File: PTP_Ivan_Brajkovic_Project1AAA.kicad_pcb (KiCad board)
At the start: 2 copper layers, 45 parts, among them J1 Screw_Terminal_01x02, SW1 SW_Push_Dual_x2, SW2 SW2, U1 LM2574N-5, U2 4027, U3 4027, U4 74LS47, U5 FYS-3911BUHR-21, U6 74LVC1G11, U7 NE555P

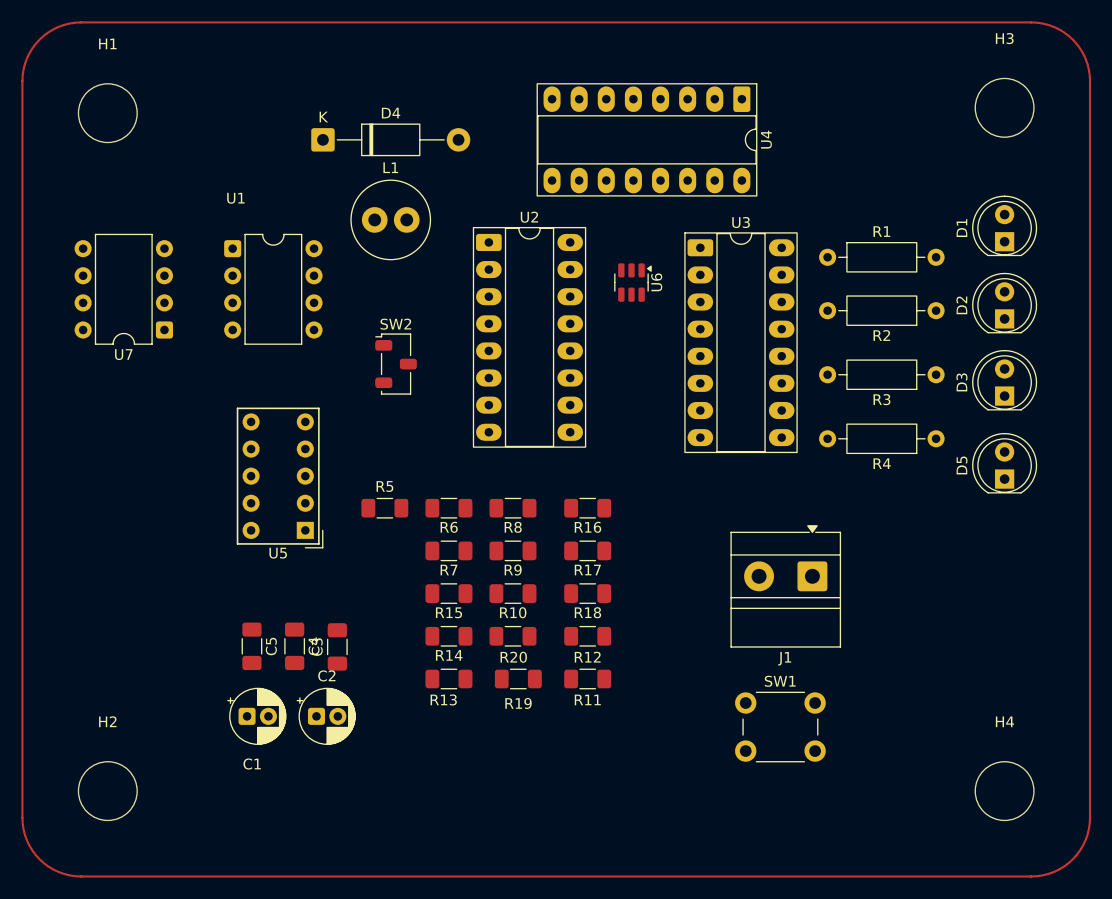
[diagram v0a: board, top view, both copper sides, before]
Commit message: lv7
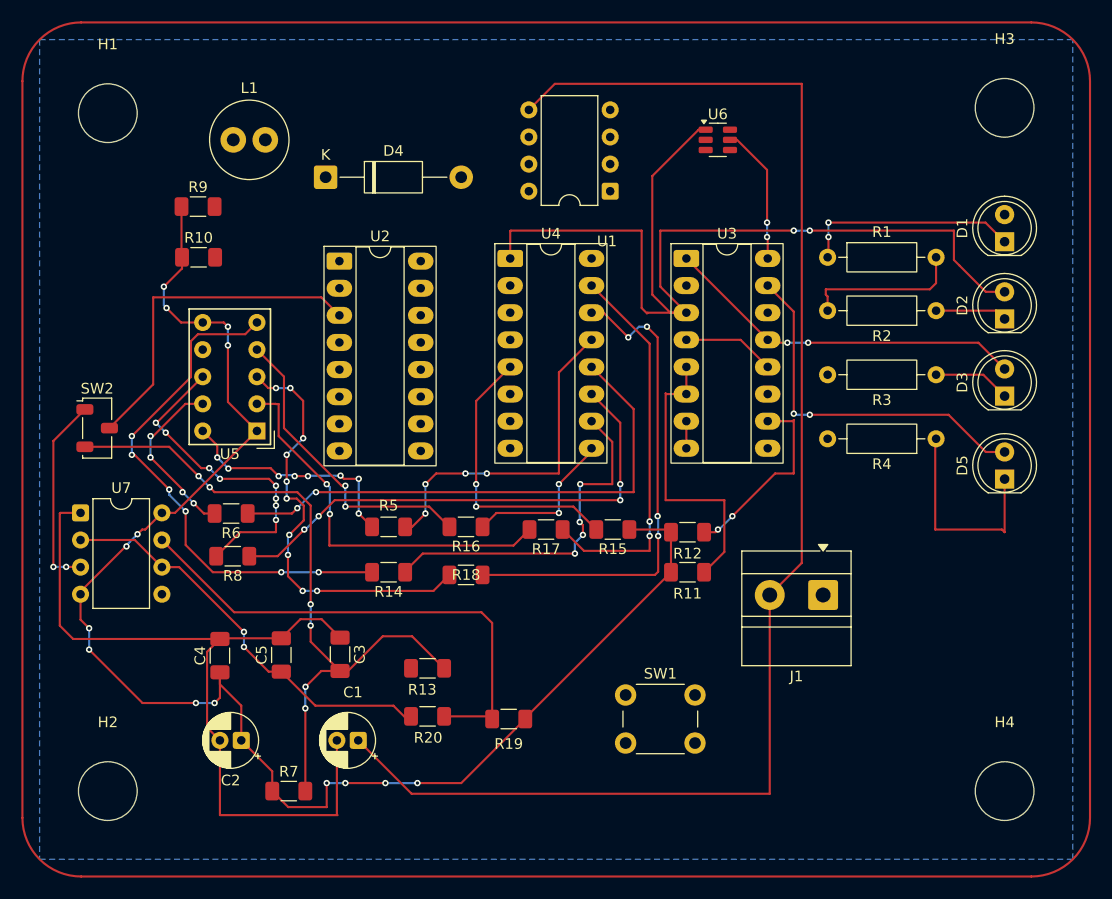
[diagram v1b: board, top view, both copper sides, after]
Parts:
- moved R9 43.7 mm to (148.4, 73.2), turned to 0 degrees
- moved R10 43.1 mm to (148.5, 78.0), turned to 0 degrees
- moved U1 35.8 mm to (187.1, 71.8), turned to 180 degrees
- moved SW2 28.6 mm to (139.0, 94.0)
- moved R7 27.0 mm to (156.9, 128.0), turned to 0 degrees
- moved R8 26.6 mm to (151.7, 106.0)
- moved U4 26.3 mm to (177.7, 78.1), turned to 0 degrees
- moved R6 20.4 mm to (151.6, 102.0)
- moved U7 18.8 mm to (137.4, 101.9), turned to 0 degrees
- moved R15 16.5 mm to (187.3, 103.5)
- moved U6 15.6 mm to (197.1, 67.0), turned to 0 degrees
- moved L1 15.2 mm to (151.8, 67.0)
- moved U2 14.1 mm to (161.7, 78.4)
- moved R11 13.7 mm to (194.3, 107.5)
- moved R12 13.5 mm to (194.3, 103.8)
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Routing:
- net +5V: track 0.00 -> 156.0 mm, vias 0 -> 16
- net VD: track 0.00 -> 134.9 mm
- net GND: track 0.00 -> 94.2 mm
- net Q1: track 0.00 -> 93.3 mm, vias 0 -> 2
- net Net-(SW2-A): track 0.00 -> 66.0 mm, vias 0 -> 6
- net Net-(U4-b): track 0.00 -> 50.3 mm, vias 0 -> 2
- net Net-(U5-D): track 0.00 -> 49.0 mm, vias 0 -> 6
- net Net-(U4-c): track 0.00 -> 48.0 mm, vias 0 -> 4
- net Net-(U7-DIS): track 0.00 -> 47.8 mm
- net Net-(U4-g): track 0.00 -> 46.5 mm, vias 0 -> 4
- net Net-(U5-G): track 0.00 -> 40.5 mm, vias 0 -> 10
- net Net-(U7-THR): track 0.00 -> 38.6 mm, vias 0 -> 2
- net Net-(U5-F): track 0.00 -> 36.7 mm, vias 0 -> 2
- net Net-(U4-f): track 0.00 -> 36.1 mm, vias 0 -> 2
- net Q3: track 0.00 -> 34.2 mm, vias 0 -> 2
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- added copper zone on B.Cu, net GND
